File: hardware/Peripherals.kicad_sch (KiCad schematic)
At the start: 2 parts

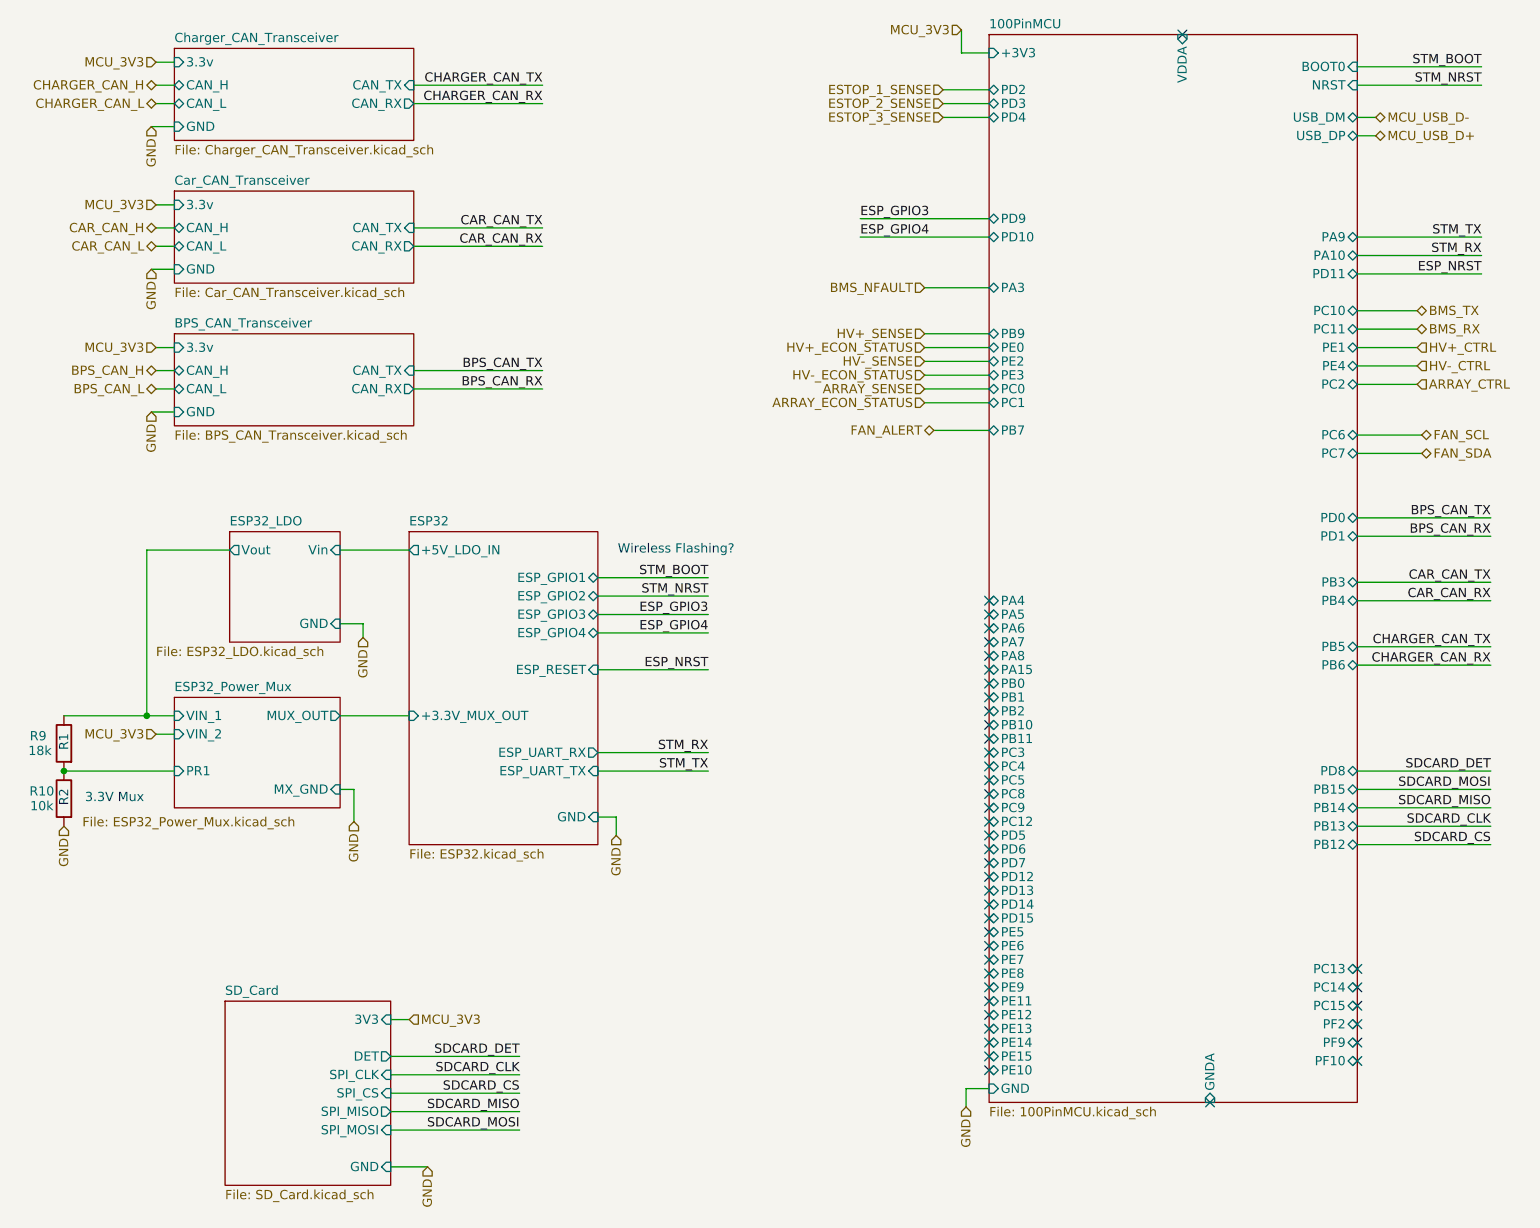
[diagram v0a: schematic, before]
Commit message: forgot to push last night
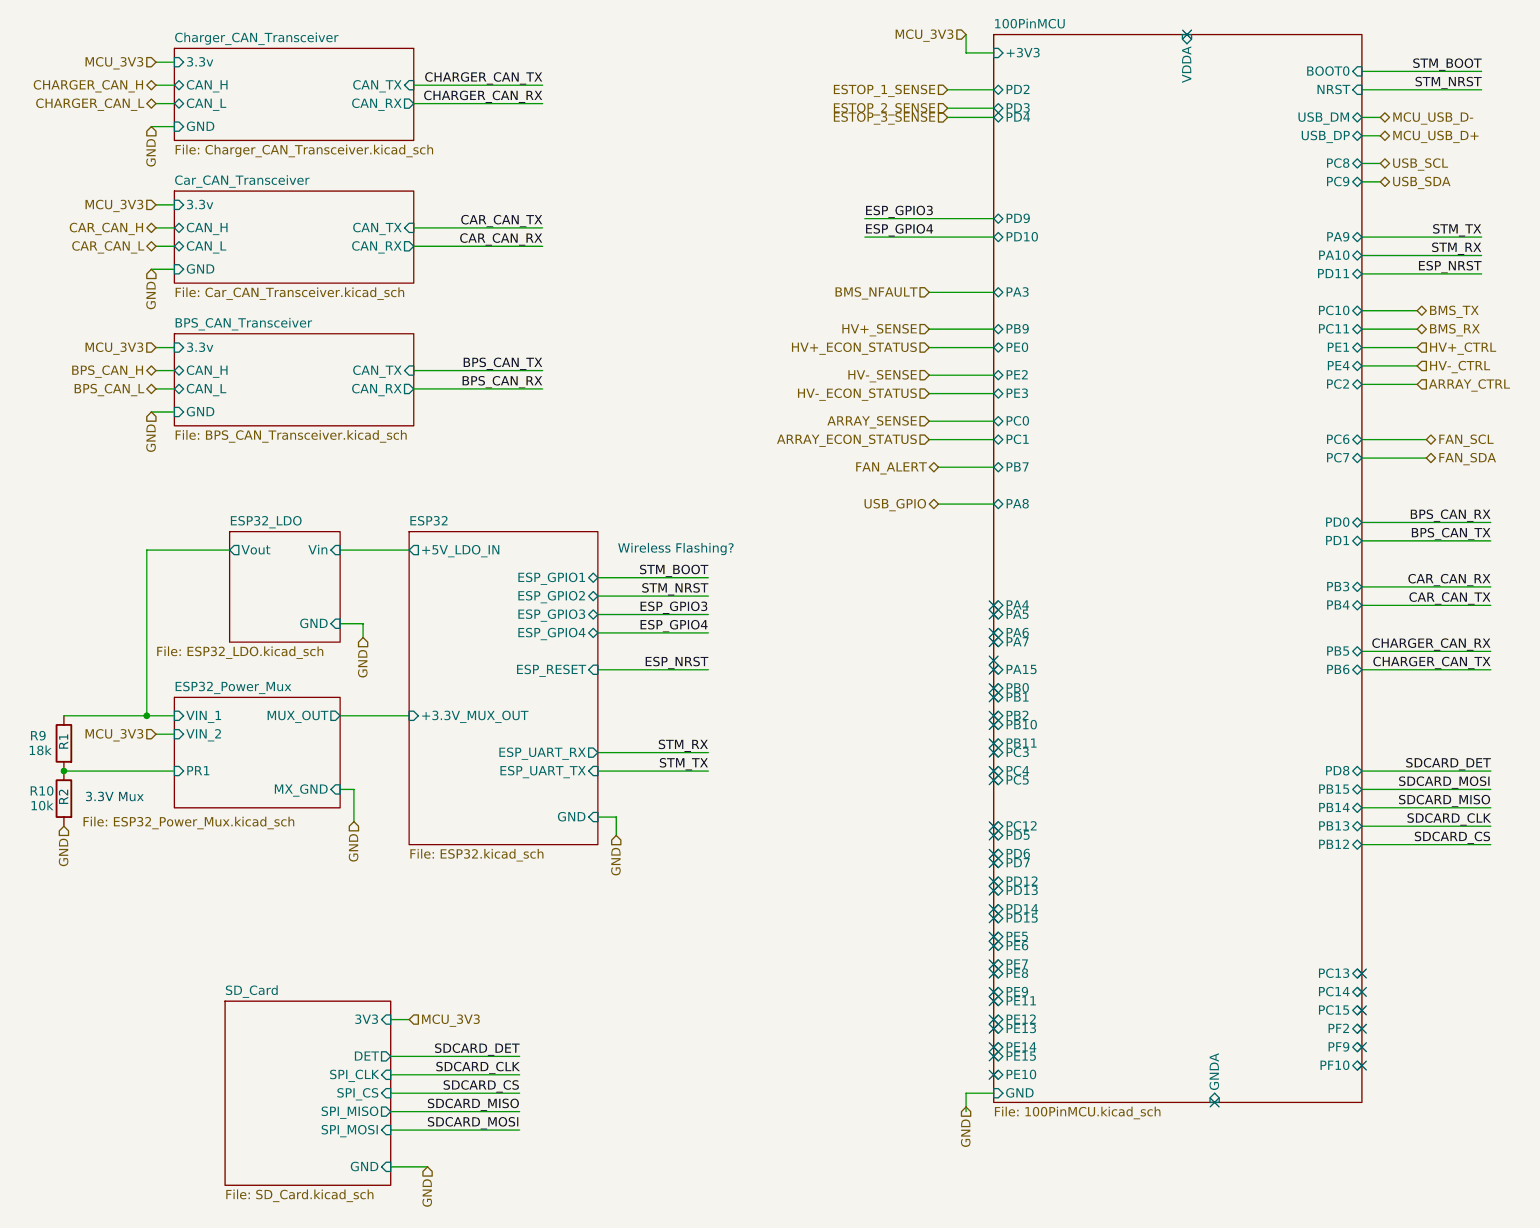
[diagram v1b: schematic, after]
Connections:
- no-connect marks 43 -> 41
